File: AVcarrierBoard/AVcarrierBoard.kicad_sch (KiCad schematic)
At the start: 16 parts, among them J1 Mech_Switch, J2 Mech_Switch, J3 MainRecov, J4 DrogRecov, J5 Staging, J6 Mech_Switch, U2 WiFi Switch, U3 EggtimerQuantum, U4 EggfinderMini/FeatherGPS, U5 Blue_Raven

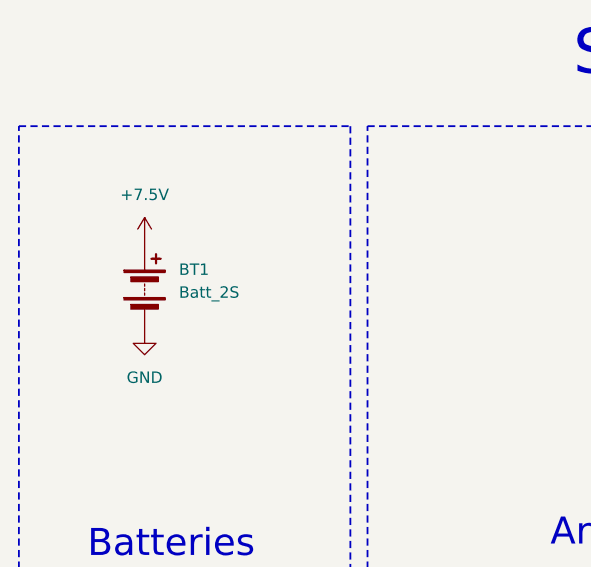
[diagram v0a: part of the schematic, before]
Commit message: final edits made, order placed
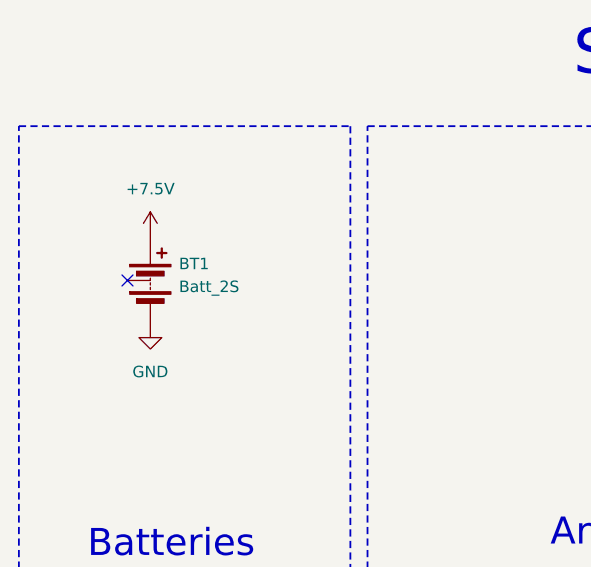
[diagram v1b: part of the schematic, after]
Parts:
- BT1: symbol Device:Battery -> COTS_boards:Battery
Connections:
- net GND: now also BT1.3 (-); no longer BT1.2 (-)
- new net: BT1.2 (middle), BT1.4 (middle)
- no-connect marks 0 -> 1
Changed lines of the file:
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@@
 (kicad_sch (version 20230121) (generator eeschema)
   (paper "A4")
+  (no_connect (at 31.75 52.07))
   (rectangle (start 86.995 154.94) (end 142.875 179.07)
     (stroke (width 0.2) (type dash))
@@
     )
   )
-  (symbol (lib_id "Device:Battery") (at 33.655 52.705 0) (unit 1)
-    (in_bom yes) (on_board yes) (dnp no) (fields_autoplaced)
-    (property "Reference" "BT1" (at 37.465 50.8635 0)
-      (effects (font (size 1.27 1.27)) (justify left))
-    )
-    (property "Value" "Batt_2S" (at 37.465 53.4035 0)
-      (effects (font (size 1.27 1.27)) (justify left))
-    )
-    (property "Footprint" "COTS_Boards:BAT_1048P" (at 33.655 51.181 90)
-      (effects (font (size 1.27 1.27)) hide)
-    )
-    (property "Datasheet" "~" (at 33.655 51.181 90)
-      (effects (font (size 1.27 1.27)) hide)
-    )
-    (pin "1")
-    (pin "2")
-    (instances
-      (project "AVcarrierBoard"
-        (path "/7d4c9aa4-eccf-4732-8f5d-af2c3b6d9138"
-          (reference "BT1") (unit 1)
-        )
-      )
-    )
-  )
-  (symbol (lib_id "Mechanical:MountingHole") (at 64.77 162.56 0) (unit 1)
-    (in_bom yes) (on_board yes) (dnp no) (fields_autoplaced)
-    (property "Reference" "H4" (at 67.31 161.29 0)
-      (effects (font (size 1.27 1.27)) (justify left))
-    )
-    (property "Value" "M3" (at 67.31 163.83 0)
-      (effects (font (size 1.27 1.27)) (justify left))
-    )
-    (property "Footprint" "MountingHole:MountingHole_3.2mm_M3_ISO14580" (at 64.77 162.56 0)
-      (effects (font (size 1.27 1.27)) hide)
-    )
-    (property "Datasheet" "~" (at 64.77 162.56 0)
-      (effects (font (size 1.27 1.27)) hide)
-    )
-    (instances
-      (project "AVcarrierBoard"
-        (path "/7d4c9aa4-eccf-4732-8f5d-af2c3b6d9138"
-          (reference "H4") (unit 1)
-        )
-      )
-    )
-  )
-  (symbol (lib_id "power:+7.5V") (at 33.655 47.625 0) (unit 1)
-    (in_bom yes) (on_board yes) (dnp no)
-    (property "Reference" "#PWR04" (at 33.655 51.435 0)
-      (effects (font (size 1.27 1.27)) hide)
-    )
-    (property "Value" "+7.5V" (at 33.655 42.545 0)
-      (effects (font (size 1.27 1.27)))
-    )
-    (property "Footprint" "" (at 33.655 47.625 0)
-      (effects (font (size 1.27 1.27)) hide)
-    )
-    (property "Datasheet" "" (at 33.655 47.625 0)
-      (effects (font (size 1.27 1.27)) hide)
-    )
-    (pin "1")
-    (instances
-      (project "AVcarrierBoard"
-        (path "/7d4c9aa4-eccf-4732-8f5d-af2c3b6d9138"
-          (reference "#PWR04") (unit 1)
-        )
-      )
-    )
-  )
-  (symbol (lib_id "Device:Battery_Cell") (at 33.655 111.125 0) (unit 1)
-    (in_bom yes) (on_board yes) (dnp no) (fields_autoplaced)
-    (property "Reference" "BT2" (at 37.465 108.0135 0)
-      (effects (font (size 1.27 1.27)) (justify left))
-    )
-    (property "Value" "Batt_1S" (at 37.465 110.5535 0)
-      (effects (font (size 1.27 1.27)) (justify left))
-    )
-    (property "Footprint" "COTS_Boards:1042P_KEY" (at 33.655 109.601 90)
-      (effects (font (size 1.27 1.27)) hide)
-    )
-    (property "Datasheet" "~" (at 33.655 109.601 90)
-      (effects (font (size 1.27 1.27)) hide)
-    )
-    (pin "1")
-    (pin "2")
-    (instances
-      (project "AVcarrierBoard"
-        (path "/7d4c9aa4-eccf-4732-8f5d-af2c3b6d9138"
-          (reference "BT2") (unit 1)
-        )
-      )
-    )
-  )
-  (symbol (lib_id "Connector:Screw_Terminal_01x04") (at 257.81 51.435 0) (unit 1)
-    (in_bom yes) (on_board yes) (dnp no) (fields_autoplaced)
-    (property "Reference" "J3" (at 260.35 51.435 0)
-      (effects (font (size 1.27 1.27)) (justify left))
-    )
-    (property "Value" "MainRecov" (at 260.35 53.975 0)
-      (effects (font (size 1.27 1.27)) (justify left))
-    )
-    (property "Footprint" "COTS_Boards:TE_282837-4-2" (at 257.81 51.435 0)
-      (effects (font (size 1.27 1.27)) hide)
-    )
-    (property "Datasheet" "~" (at 257.81 51.435 0)
-      (effects (font (size 1.27 1.27)) hide)
-    )
+  (symbol (lib_id "COTS_boards:Battery") (at 34.29 52.07 0) (unit 1)
+    (in_bom yes) (on_board yes) (dnp no) (fields_autoplaced)
+    (property "Reference" "BT1" (at 37.465 50.2285 0)
+      (effects (font (size 1.27 1.27)) (justify left))
+    )
+    (property "Value" "Batt_2S" (at 37.465 52.7685 0)
+      (effects (font (size 1.27 1.27)) (justify left))
+    )
+    (property "Footprint" "COTS_Boards:BAT_1048P" (at 34.29 50.546 90)
+      (effects (font (size 1.27 1.27)) hide)
+    )
+    (property "Datasheet" "~" (at 34.29 50.546 90)
+      (effects (font (size 1.27 1.27)) hide)
+    )
+    (pin "1")
     (pin "4")
     (pin "3")
     (pin "2")
+    (instances
+      (project "AVcarrierBoard"
+        (path "/7d4c9aa4-eccf-4732-8f5d-af2c3b6d9138"
+          (reference "BT1") (unit 1)
+        )
+      )
+    )
+  )
+  (symbol (lib_id "Mechanical:MountingHole") (at 64.77 162.56 0) (unit 1)
+    (in_bom yes) (on_board yes) (dnp no) (fields_autoplaced)
+    (property "Reference" "H4" (at 67.31 161.29 0)
+      (effects (font (size 1.27 1.27)) (justify left))
+    )
+    (property "Value" "M3" (at 67.31 163.83 0)
+      (effects (font (size 1.27 1.27)) (justify left))
+    )
+    (property "Footprint" "MountingHole:MountingHole_3.2mm_M3_ISO14580" (at 64.77 162.56 0)
+      (effects (font (size 1.27 1.27)) hide)
+    )
+    (property "Datasheet" "~" (at 64.77 162.56 0)
+      (effects (font (size 1.27 1.27)) hide)
+    )
+    (instances
+      (project "AVcarrierBoard"
+        (path "/7d4c9aa4-eccf-4732-8f5d-af2c3b6d9138"
+          (reference "H4") (unit 1)
+        )
+      )
+    )
+  )
+  (symbol (lib_id "power:+7.5V") (at 34.29 46.99 0) (unit 1)
+    (in_bom yes) (on_board yes) (dnp no)
+    (property "Reference" "#PWR04" (at 34.29 50.8 0)
+      (effects (font (size 1.27 1.27)) hide)
+    )
+    (property "Value" "+7.5V" (at 34.29 41.91 0)
+      (effects (font (size 1.27 1.27)))
+    )
+    (property "Footprint" "" (at 34.29 46.99 0)
+      (effects (font (size 1.27 1.27)) hide)
+    )
+    (property "Datasheet" "" (at 34.29 46.99 0)
+      (effects (font (size 1.27 1.27)) hide)
+    )
+    (pin "1")
+    (instances
+      (project "AVcarrierBoard"
+        (path "/7d4c9aa4-eccf-4732-8f5d-af2c3b6d9138"
+          (reference "#PWR04") (unit 1)
+        )
+      )
+    )
+  )
+  (symbol (lib_id "Device:Battery_Cell") (at 33.655 111.125 0) (unit 1)
+    (in_bom yes) (on_board yes) (dnp no) (fields_autoplaced)
+    (property "Reference" "BT2" (at 37.465 108.0135 0)
+      (effects (font (size 1.27 1.27)) (justify left))
+    )
+    (property "Value" "Batt_1S" (at 37.465 110.5535 0)
+      (effects (font (size 1.27 1.27)) (justify left))
+    )
+    (property "Footprint" "COTS_Boards:1042P_KEY" (at 33.655 109.601 90)
+      (effects (font (size 1.27 1.27)) hide)
+    )
+    (property "Datasheet" "~" (at 33.655 109.601 90)
+      (effects (font (size 1.27 1.27)) hide)
+    )
+    (pin "1")
+    (pin "2")
+    (instances
+      (project "AVcarrierBoard"
+        (path "/7d4c9aa4-eccf-4732-8f5d-af2c3b6d9138"
+          (reference "BT2") (unit 1)
+        )
+      )
+    )
+  )
+  (symbol (lib_id "Connector:Screw_Terminal_01x04") (at 257.81 51.435 0) (unit 1)
+    (in_bom yes) (on_board yes) (dnp no) (fields_autoplaced)
+    (property "Reference" "J3" (at 260.35 51.435 0)
+      (effects (font (size 1.27 1.27)) (justify left))
+    )
+    (property "Value" "MainRecov" (at 260.35 53.975 0)
+      (effects (font (size 1.27 1.27)) (justify left))
+    )
+    (property "Footprint" "COTS_Boards:TE_282837-4-2" (at 257.81 51.435 0)
+      (effects (font (size 1.27 1.27)) hide)
+    )
+    (property "Datasheet" "~" (at 257.81 51.435 0)
+      (effects (font (size 1.27 1.27)) hide)
+    )
+    (pin "4")
+    (pin "3")
+    (pin "2")
     (pin "1")
     (instances
@@
     )
   )
-  (symbol (lib_id "power:GND") (at 33.655 57.785 0) (unit 1)
-    (in_bom yes) (on_board yes) (dnp no) (fields_autoplaced)
-    (property "Reference" "#PWR01" (at 33.655 64.135 0)
-      (effects (font (size 1.27 1.27)) hide)
-    )
-    (property "Value" "GND" (at 33.655 62.865 0)
-      (effects (font (size 1.27 1.27)))
-    )
-    (property "Footprint" "" (at 33.655 57.785 0)
-      (effects (font (size 1.27 1.27)) hide)
-    )
-    (property "Datasheet" "" (at 33.655 57.785 0)
-      (effects (font (size 1.27 1.27)) hide)
-    )
+  (symbol (lib_id "power:GND") (at 34.29 57.15 0) (unit 1)
+    (in_bom yes) (on_board yes) (dnp no) (fields_autoplaced)
+    (property "Reference" "#PWR01" (at 34.29 63.5 0)
+      (effects (font (size 1.27 1.27)) hide)
+    )
+    (property "Value" "GND" (at 34.29 62.23 0)
+      (effects (font (size 1.27 1.27)))
+    )
+    (property "Footprint" "" (at 34.29 57.15 0)
+      (effects (font (size 1.27 1.27)) hide)
+    )
+    (property "Datasheet" "" (at 34.29 57.15 0)
+      (effects (font (size 1.27 1.27)) hide)
+    )
